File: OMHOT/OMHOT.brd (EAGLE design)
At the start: 103 x 86.5 mm, 60 parts, among them J1 PTDA_1.5_4-PH_5.0, J3 8PIN_CON_AMP, J4 TERMINAL_2PIN, J5 TERMINAL_2PIN, J6 TERMINAL_2PIN, J7 TERMINAL_2PIN, J8 TERMINAL_2PIN, J9 TERMINAL_2PIN, K1 H550, K2 H550, K3 H550, K4 H550, K5 H550, K6 H550, K7 H550, K8 H550, U1 OKI-78SR, U2 MAX481CSA, U3 PIC18F4XK80, U4 ULN2803A, U5 ULN2803A, Y1 10MHz

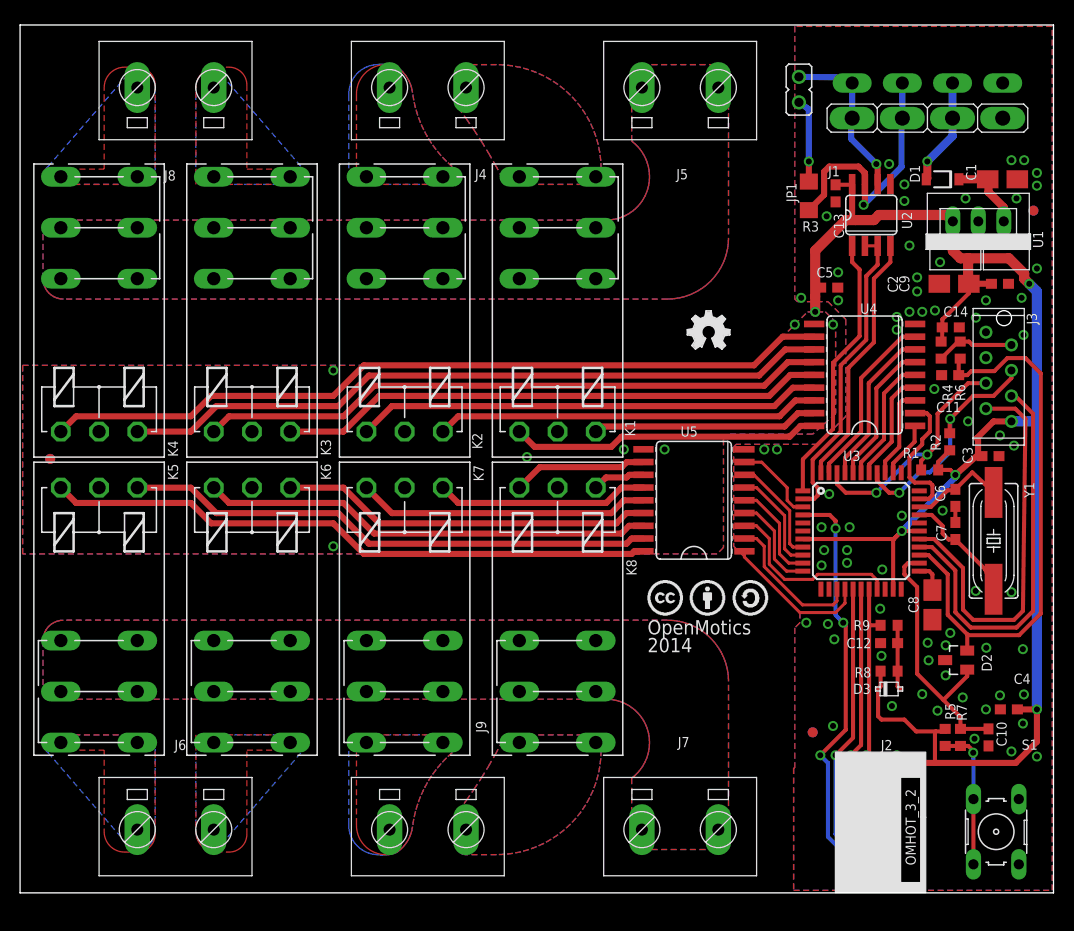
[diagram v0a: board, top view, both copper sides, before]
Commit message: Added my version and firmware
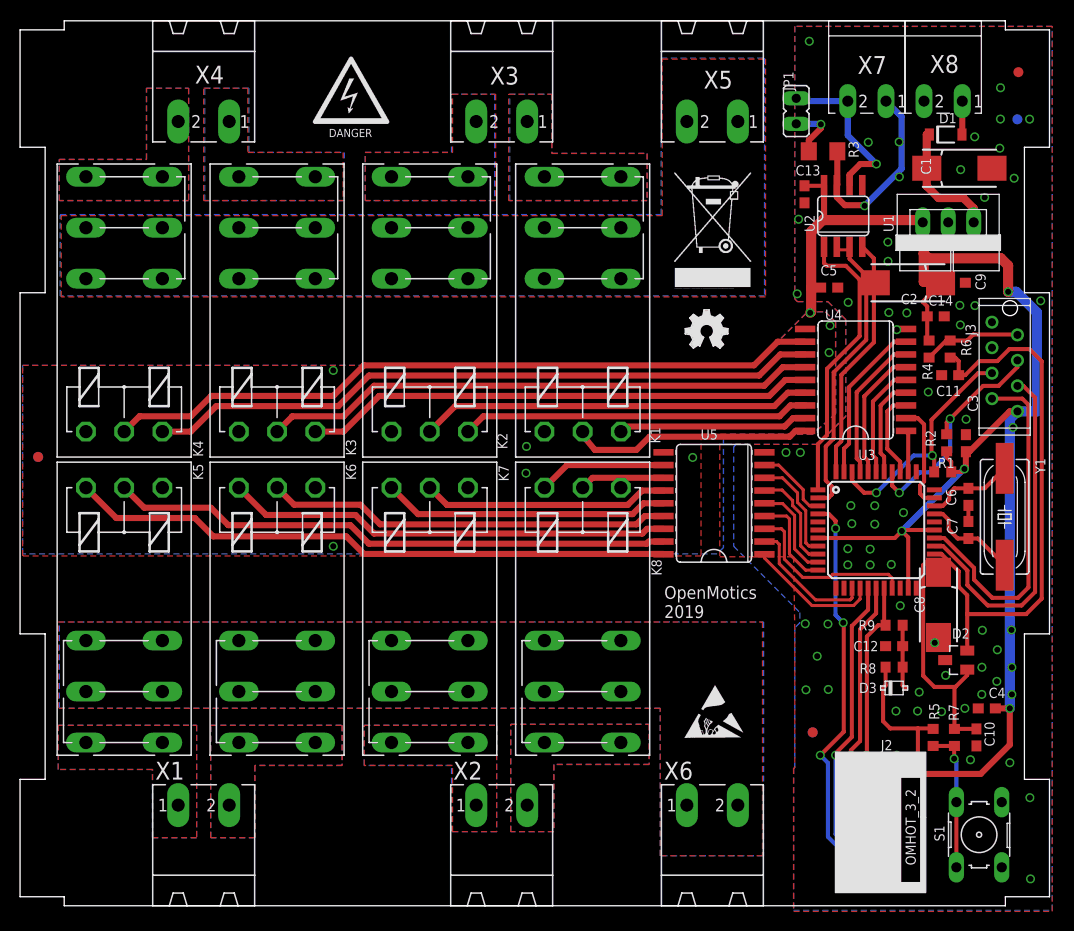
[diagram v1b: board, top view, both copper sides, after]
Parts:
- removed J1: PTDA_1.5_4-PH_5.0, OpenMotics:PTDA_1.5_X-PH_5.0
- removed J4, J5, J6, J7, J8, J9: TERMINAL_2PIN, OpenMotics:2PIN_TERMINAL_7.6MM
- removed U$7: CC_BY_SA, OpenMotics:CC_BY_SA
- added U$10: (no value), ruben:ESD
- added U$11: (no value), ruben:HIGH-VOLTAGE
- added U$8: DISPOSAL-SYMBOL, ruben:DISPOSAL
- added X1, X2, X3, X4, X5, X6: CIM029M5, ruben:CIM029M5
- added X7, X8: CTM029MT, ruben:CTM029MT
- C1, C2, C8: device resistor:A3216-18W -> resistor:085CS_1AR
- J2: device OpenMotics:PROG_CON_WITH_VERSION -> ruben:PROG_CON_WITH_VERSION
- J3: device OpenMotics:8PIN_CON_AMP -> ruben:8PIN_CON_AMP
- JP1: device jumper:JP1S -> jumper:JP1
- U2: device maxim:SO08 -> ruben:SO08
- moved U$4 105.7 mm to (104.2, -1.75)
- moved U$3 13.9 mm to (99.5, 81.8)
- moved U$1 9.24 mm to (99.4, 77.1)
- moved R3 4.66 mm to (80.0, 73.9), turned to 180 degrees
- moved C2 4.60 mm to (88.5, 60.8)
- moved D1 4.47 mm to (92.3, 75.6), turned to 0 degrees
- moved C1 4.44 mm to (93.6, 72.2)
- moved C9 4.30 mm to (93.4, 60.8)
- moved C13 3.10 mm to (78.2, 69.6)
- moved U1 3.00 mm to (95.0, 66.8)
- moved U2 2.80 mm to (82.0, 67.5)
- moved C3 2.77 mm to (94.3, 44.8), turned to 90 degrees
- moved Y1 2.64 mm to (98.1, 37.5)
- moved K4 2.50 mm to (10.4, 53.6)
- moved K5 2.50 mm to (10.4, 32.8)
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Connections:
- net +5V: now also K1.1, K2.1, K3.1, K4.1, K5.1, K6.1, K7.1, K8.1; no longer K1.3, K2.3, K3.3, K4.3, K5.3, K6.3, K7.3, K8.3
- net 0V: now also X8.2; no longer J1.P$4, J1.P$8
- net 12V_IN: now also X8.1; no longer J1.P$3, J1.P$7
- net N$1: now also X1.1; no longer J6.P$2
- net N$10: now also X2.1; no longer J9.P$2
- net N$11: now also X2.2; no longer J9.P$1
- net N$12: now also X5.1, X5.2; no longer J5.P$1, J5.P$2
- net N$13: now also X3.2; no longer J4.P$1
- net N$15: now also K2.3; no longer K2.1
- net N$17: now also K1.3; no longer K1.1
- net N$19: now also K5.3; no longer K5.1
- net N$20: now also X6.1, X6.2; no longer J7.P$1, J7.P$2
- net N$22: now also K6.3; no longer K6.1
- net N$24: now also K7.3; no longer K7.1
- net N$26: now also K8.3; no longer K8.1
- net N$3: now also X4.1; no longer J8.P$2
- net N$4: now also X4.2; no longer J8.P$1
- net N$5: now also X1.2; no longer J6.P$1
- net N$6: now also K4.3; no longer K4.1
- net N$8: now also X3.1; no longer J4.P$2
- net N$9: now also K3.3; no longer K3.1
- net RS485_A: now also X7.2; no longer J1.P$1, J1.P$5
- net RS485_B: now also X7.1; no longer J1.P$2, J1.P$6
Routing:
- net N$15: track 46.4 -> 39.0 mm
- net N$9: track 62.7 -> 55.3 mm
- net N$6: track 79.0 -> 71.6 mm
- net 12V_IN: track 10.7 -> 3.68 mm, vias 1 -> 0
- net N$17: track 30.9 -> 24.0 mm
- net RS485_B: track 26.2 -> 20.4 mm
- net STAT1: track 40.0 -> 35.1 mm
- net STAT2: track 40.3 -> 35.5 mm
- net 12V: track 7.72 -> 12.4 mm
- net N$16: track 38.3 -> 34.7 mm
- net N$14: track 54.6 -> 51.0 mm
- net N$7: track 70.9 -> 67.2 mm
- net +5V: track 180.8 -> 177.4 mm
- net N$24: track 21.3 -> 24.6 mm
- net N$18: track 22.5 -> 19.2 mm
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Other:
- board size 103 x 86.5 mm -> 102.6 x 88.2 mm
- board text added: "OpenMotics 2019"
